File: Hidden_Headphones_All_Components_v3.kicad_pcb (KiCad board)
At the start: 2 copper layers, 32 x 45 mm, 14 parts, among them SW1 POWER, SW2 VOL+, SW3 VOL-, SW4 PLAY, U1_L ESP32_L, U1_R ESP32_R, U2_DAC PCM5102A, U3_TP4056 TP4056

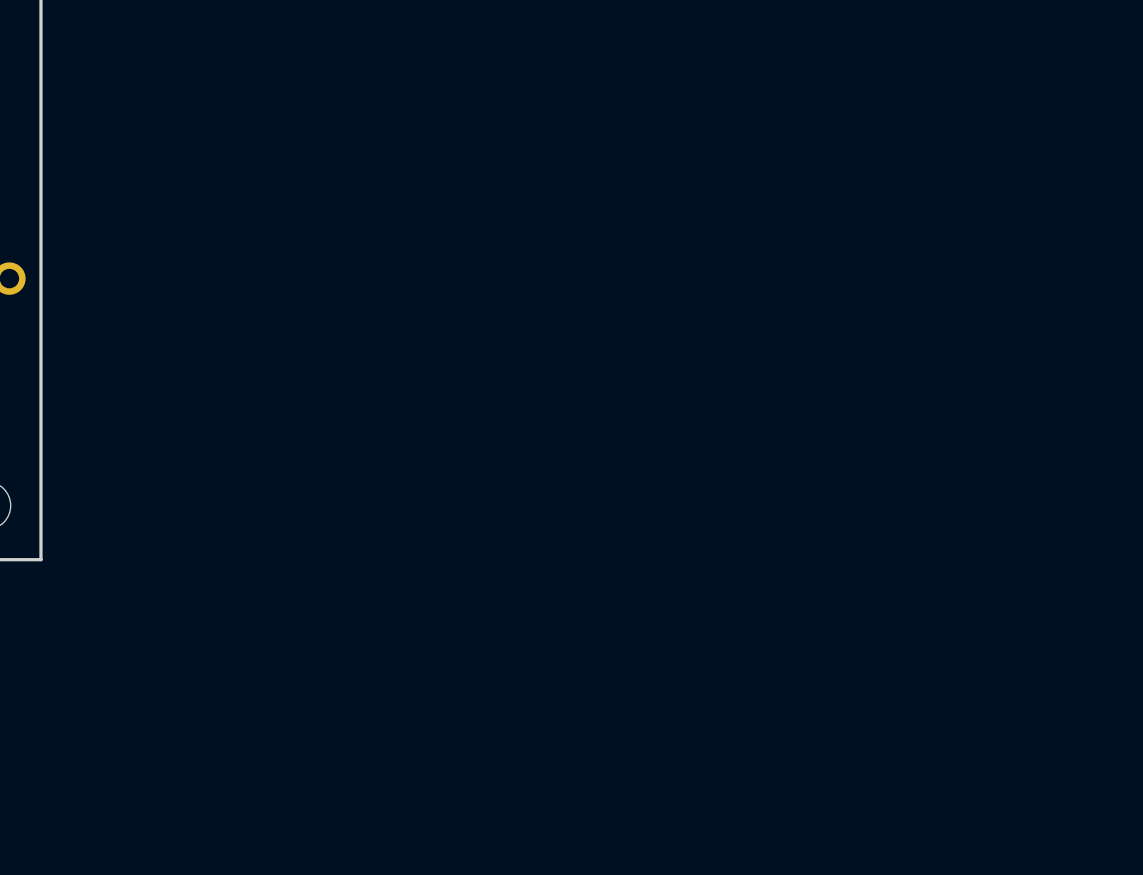
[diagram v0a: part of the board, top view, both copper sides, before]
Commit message: worked on pcb
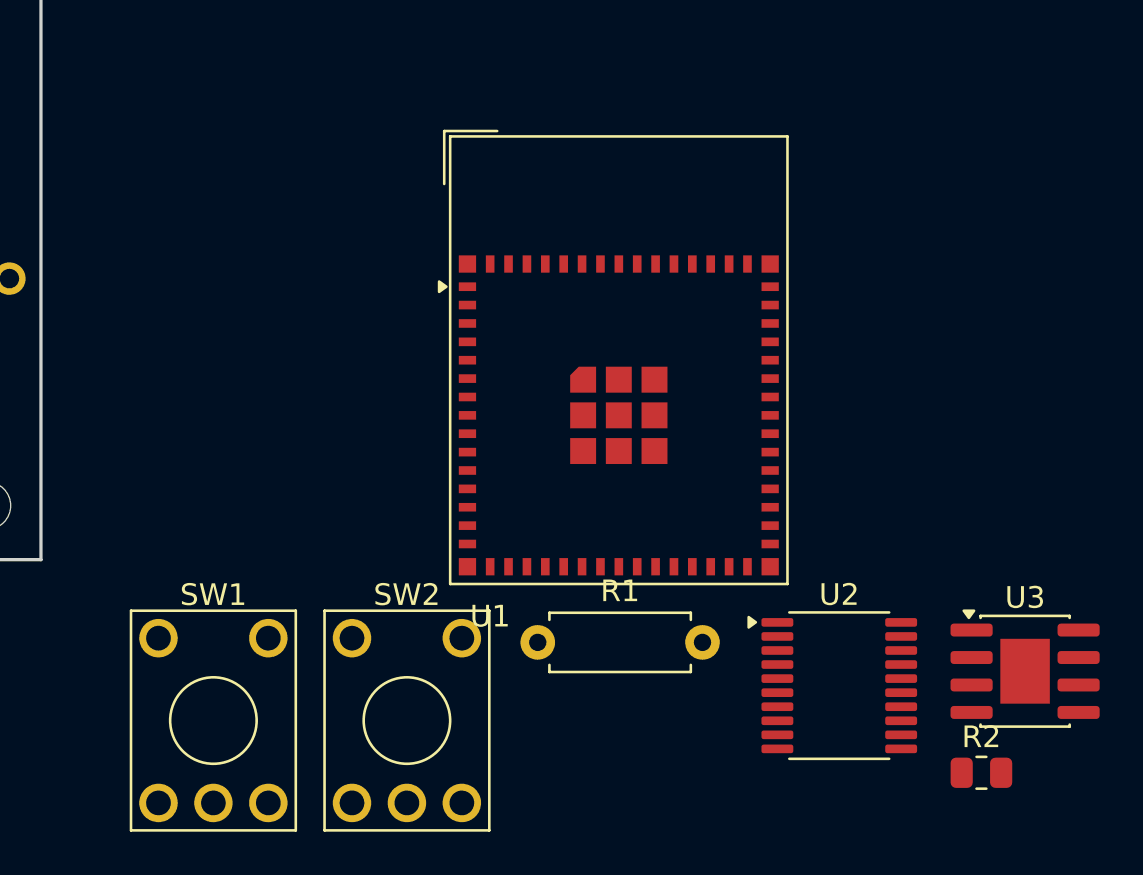
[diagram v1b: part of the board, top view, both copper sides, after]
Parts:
- added R1: 1.2kΩ, Resistor_THT:R_Axial_DIN0207_L6.3mm_D2.5mm_P7.62mm_Horizontal, F.Cu at (55.0, 48.8)
- added R2: 10kΩ, Resistor_SMD:R_0805_2012Metric, F.Cu at (75.5, 54.9)
- added SW1: SW_Push, Button_Switch_THT:KSA_Tactile_SPST, F.Cu at (37.4, 48.6)
- added SW2: SW_Push, Button_Switch_THT:KSA_Tactile_SPST, F.Cu at (46.4, 48.6)
- added U1: ESP32-S3-MINI-1, RF_Module:ESP32-S2-MINI-1, F.Cu at (58.7, 35.8)
- added U2: PCM5102A, Package_SO:TSSOP-20_4.4x6.5mm_P0.65mm, F.Cu at (68.9, 50.8)
- added U3: TP4056-42-ESOP8, Package_SO:SOIC-8-1EP_3.9x4.9mm_P1.27mm_EP2.29x3mm, F.Cu at (77.5, 50.2)
